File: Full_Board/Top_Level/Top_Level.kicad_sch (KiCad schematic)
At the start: 29 parts

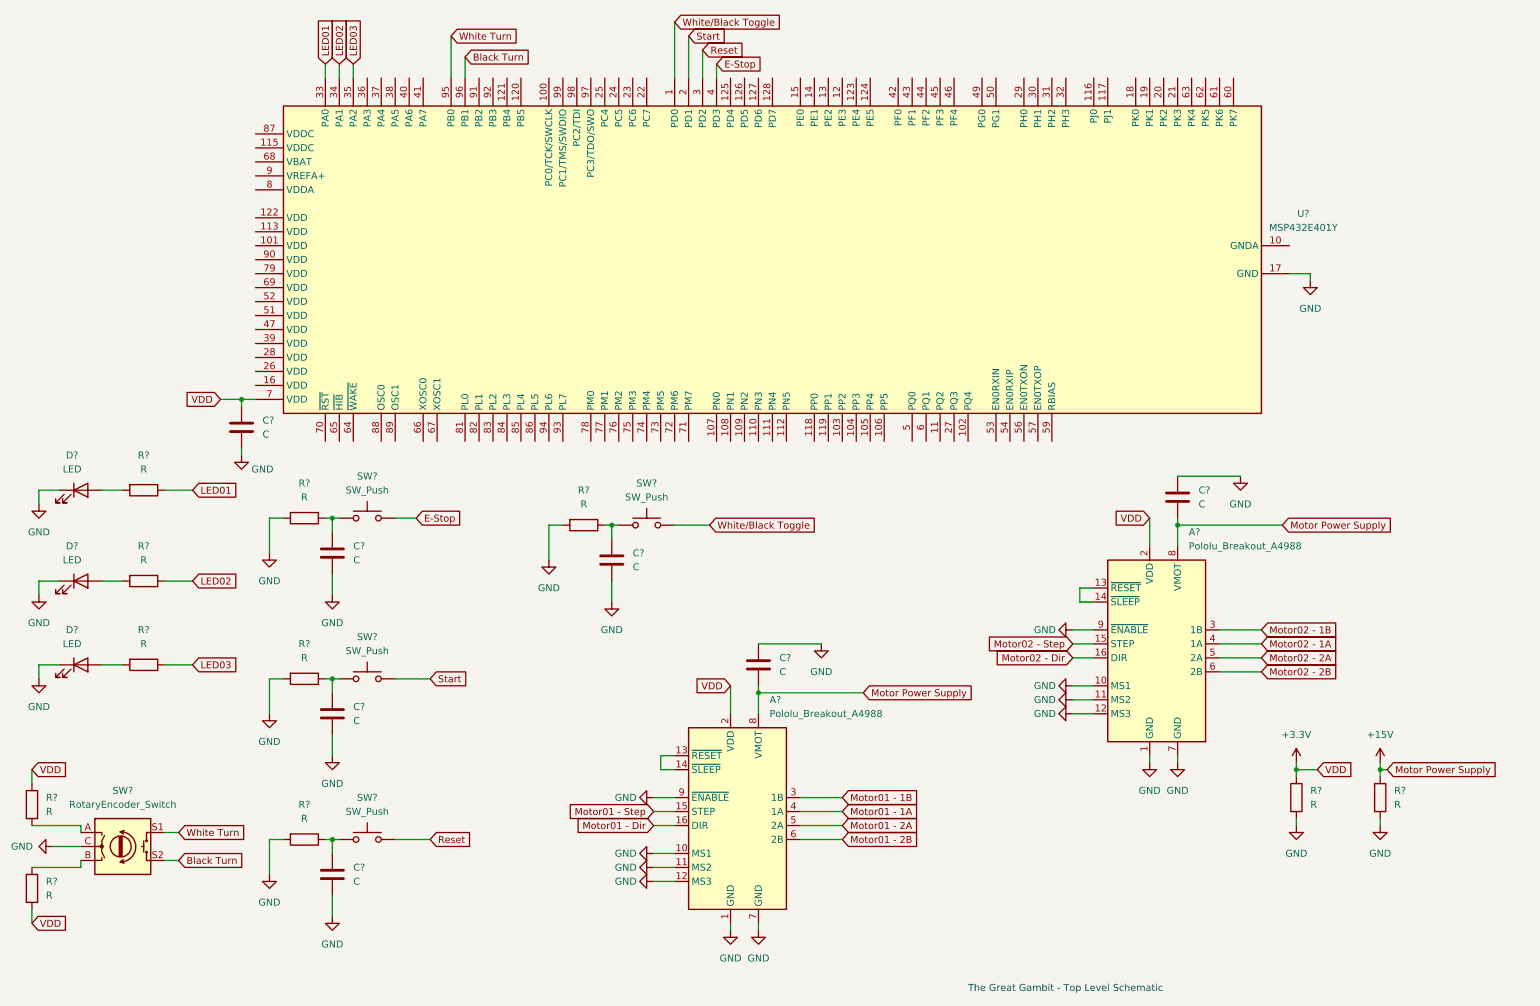
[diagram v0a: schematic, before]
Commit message: Add files via upload
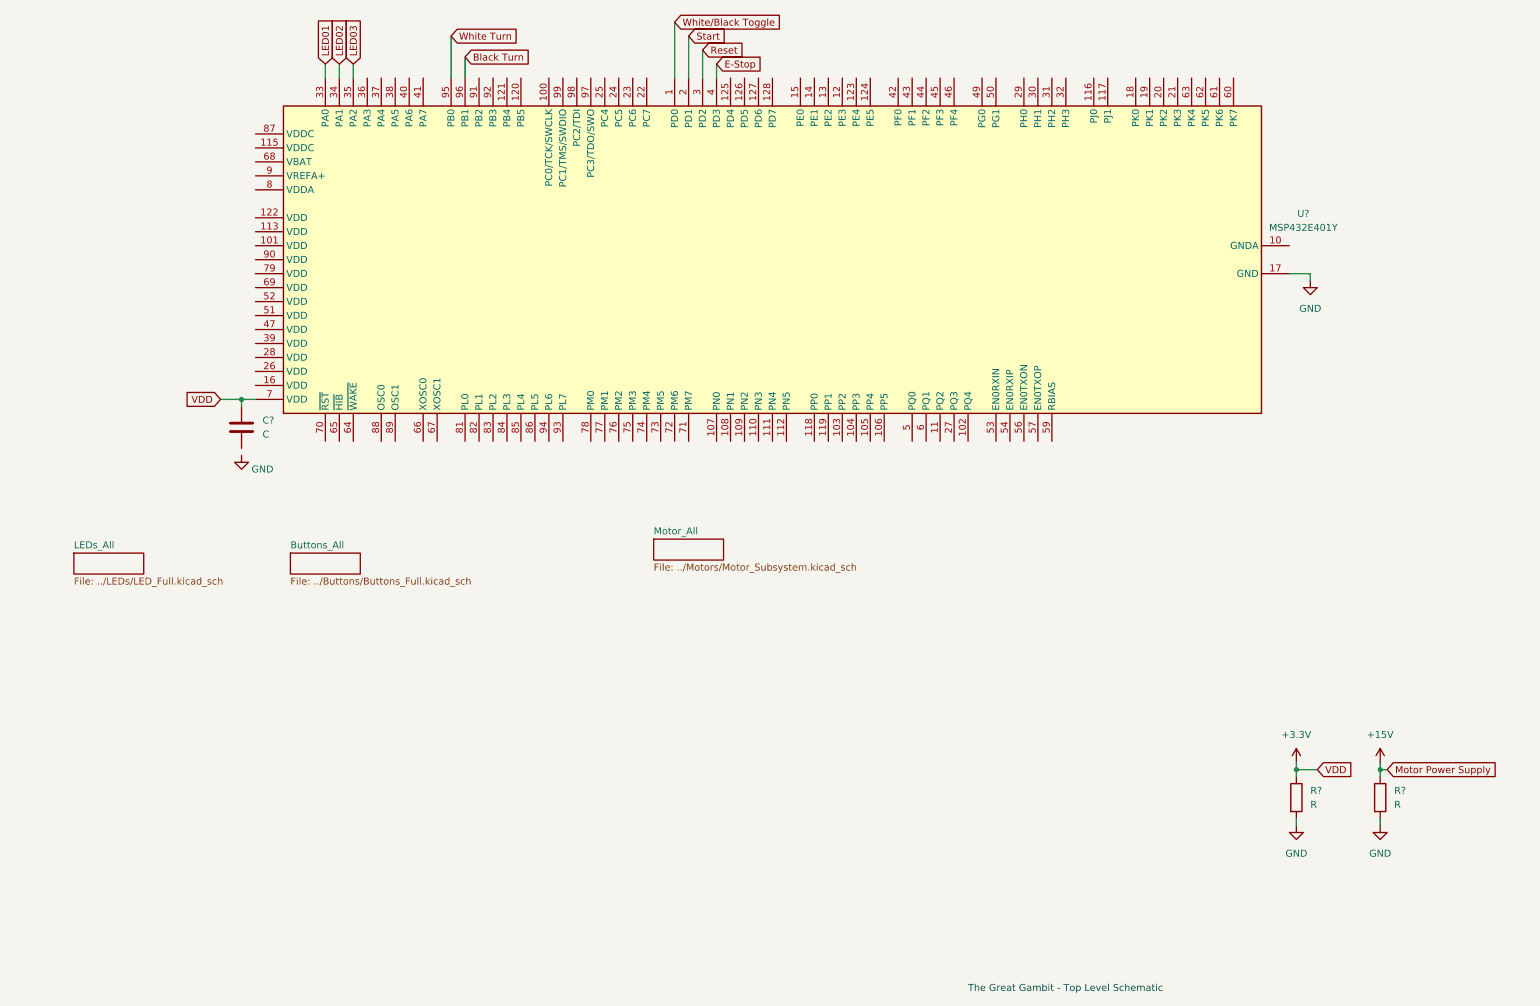
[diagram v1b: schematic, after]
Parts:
- removed A? (x2): Pololu_Breakout_A4988, Module:Pololu_Breakout-16_15.2x20.3mm, symbol Driver_Motor:Pololu_Breakout_A4988
- removed C? (x6): C, symbol Device:C
- removed D? (x3): LED, symbol Device:LED
- removed R? (x9): R, symbol Device:R
- removed SW? (x4): SW_Push, symbol Switch:SW_Push
- removed SW?: RotaryEncoder_Switch, symbol Device:RotaryEncoder_Switch
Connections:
- net GND: no longer C?.2
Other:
- added sheet Buttons_All (../Buttons/Buttons_Full.kicad_sch)
- added sheet LEDs_All (../LEDs/LED_Full.kicad_sch)
- added sheet Motor_All (../Motors/Motor_Subsystem.kicad_sch)
